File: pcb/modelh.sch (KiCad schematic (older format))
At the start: 39 parts, among them J1 USB_B, J2 Conn_01x16, J3 Conn_01x08, J4 Conn_01x04, J5 Conn_02x03_Odd_Even, J6 Conn_02x05_Odd_Even, SW1 SW_Push, U1 STM32F103C8Tx, U2 AMS1117-3.3, Y1 8MHz, Y2 32.768KHz

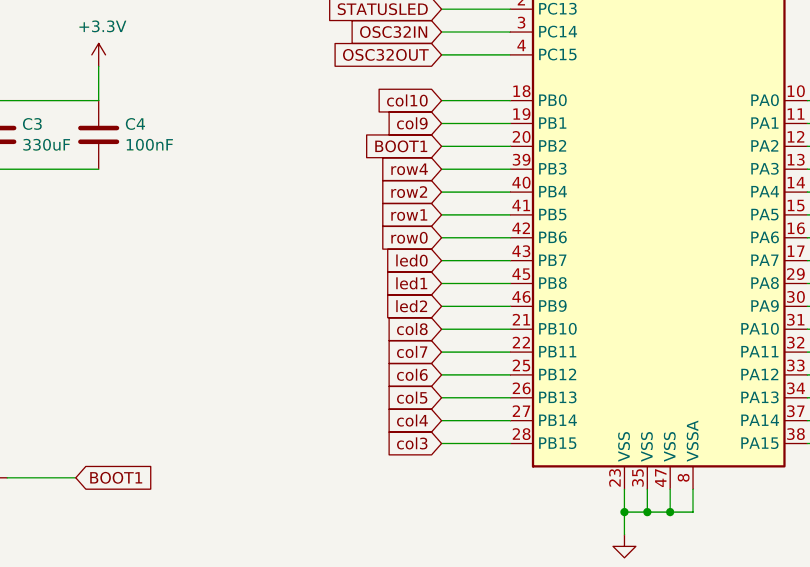
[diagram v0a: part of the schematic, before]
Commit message: WIP
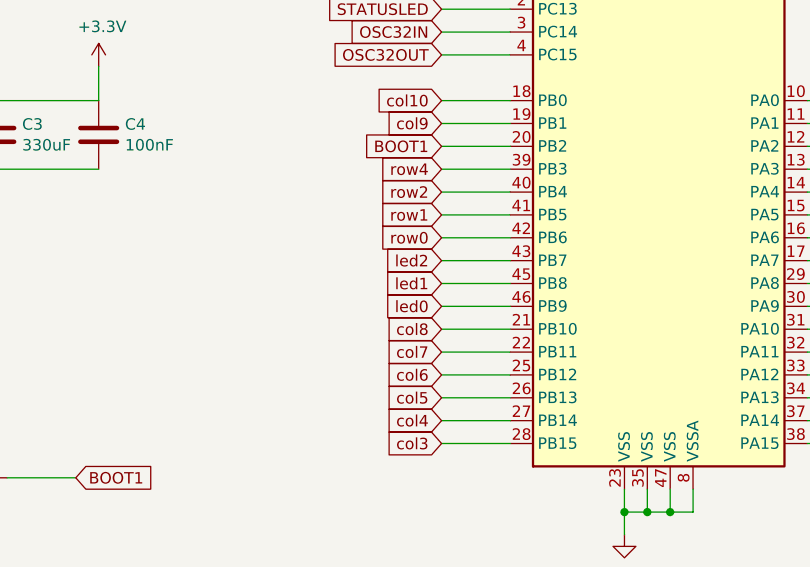
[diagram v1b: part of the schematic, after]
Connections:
- net led0: now also U1.46 (PB9); no longer U1.43 (PB7)
- net led2: now also U1.43 (PB7); no longer U1.46 (PB9)
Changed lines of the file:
@@
 	6400 4500 6700 4500
 Wire Wire Line
+	4800 4200 5100 4200
+Wire Wire Line
+	5100 4300 4800 4300
+Wire Wire Line
 	4800 4400 5100 4400
-Wire Wire Line
-	5100 4300 4800 4300
-Wire Wire Line
-	4800 4200 5100 4200
 Wire Wire Line
 	6700 3500 6400 3500
@@
 Text GLabel 4800 4100 0    50   Input ~ 0
 row0
-Text GLabel 4800 4200 0    50   Input ~ 0
+Text GLabel 4800 4400 0    50   Input ~ 0
 led0
 Text GLabel 4800 4300 0    50   Input ~ 0
 led1
-Text GLabel 4800 4400 0    50   Input ~ 0
+Text GLabel 4800 4200 0    50   Input ~ 0
 led2
 Text GLabel 4800 4500 0    50   Input ~ 0
